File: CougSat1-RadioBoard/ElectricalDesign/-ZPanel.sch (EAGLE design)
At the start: 28 parts, among them J1 High Gain Antenna, J2 Deployables, J3 High Gain +, J4 ADCS, J5 Flap +X, J6 Flap -X, J7 Flap +Y, J8 Flap -Y, U1 LTC2499, U2 MCP1501-18

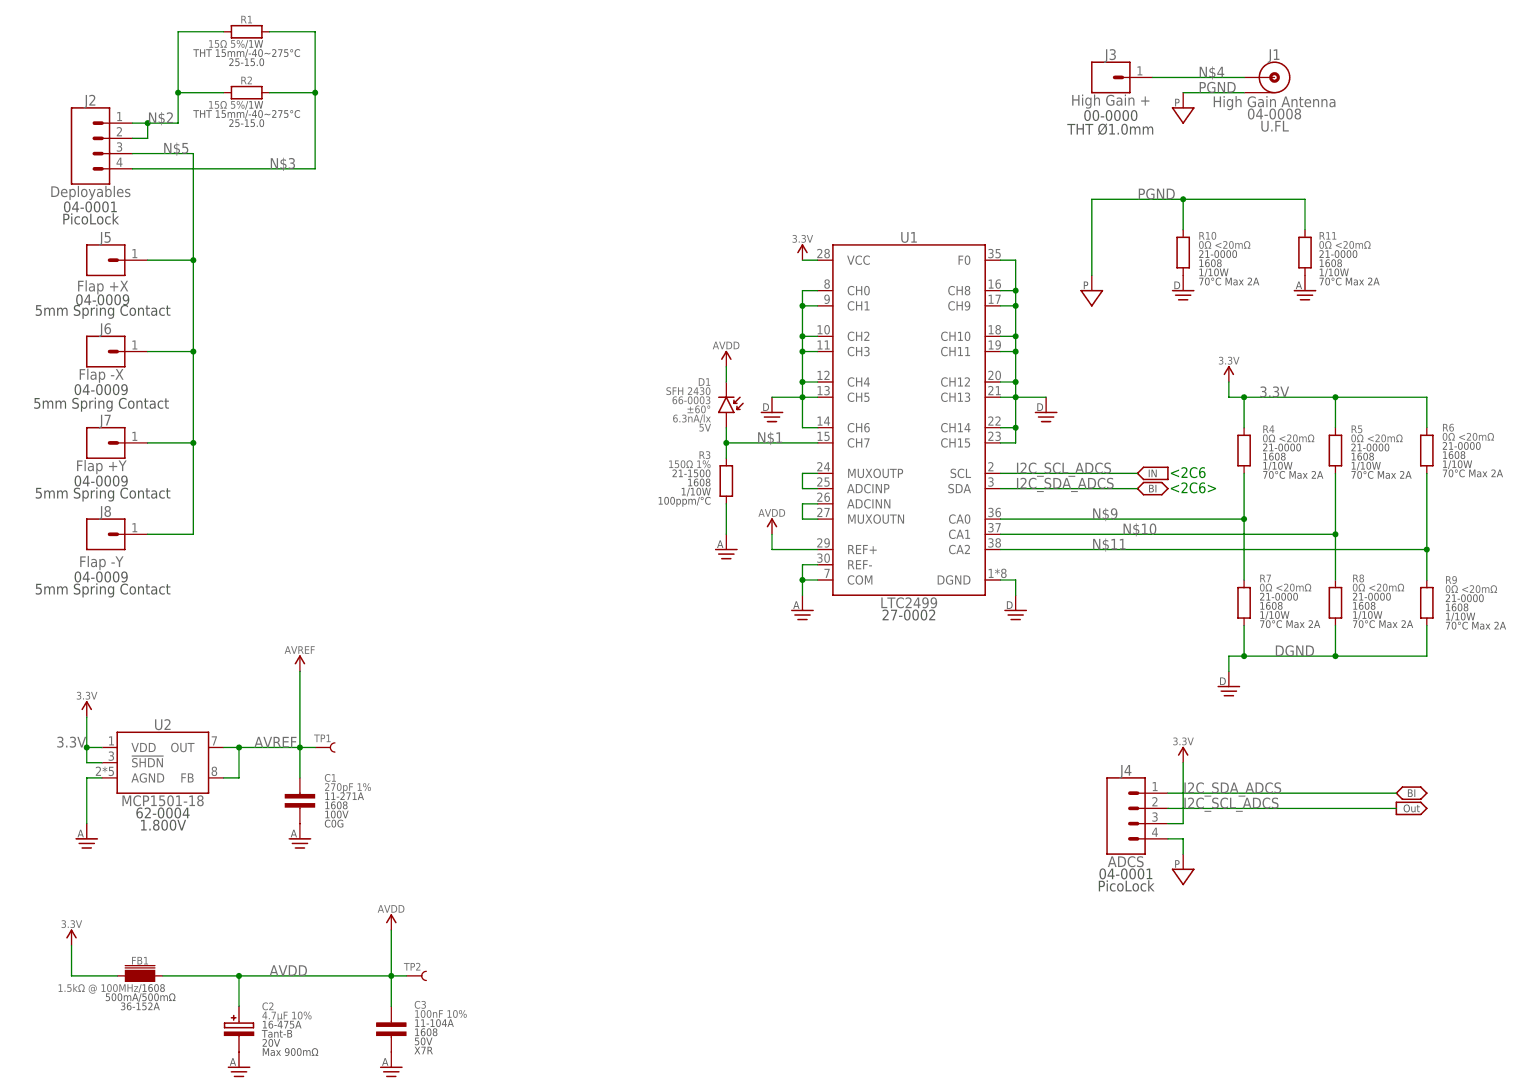
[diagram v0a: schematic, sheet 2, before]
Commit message: Update -ZPanel.sch
Ready for re-review
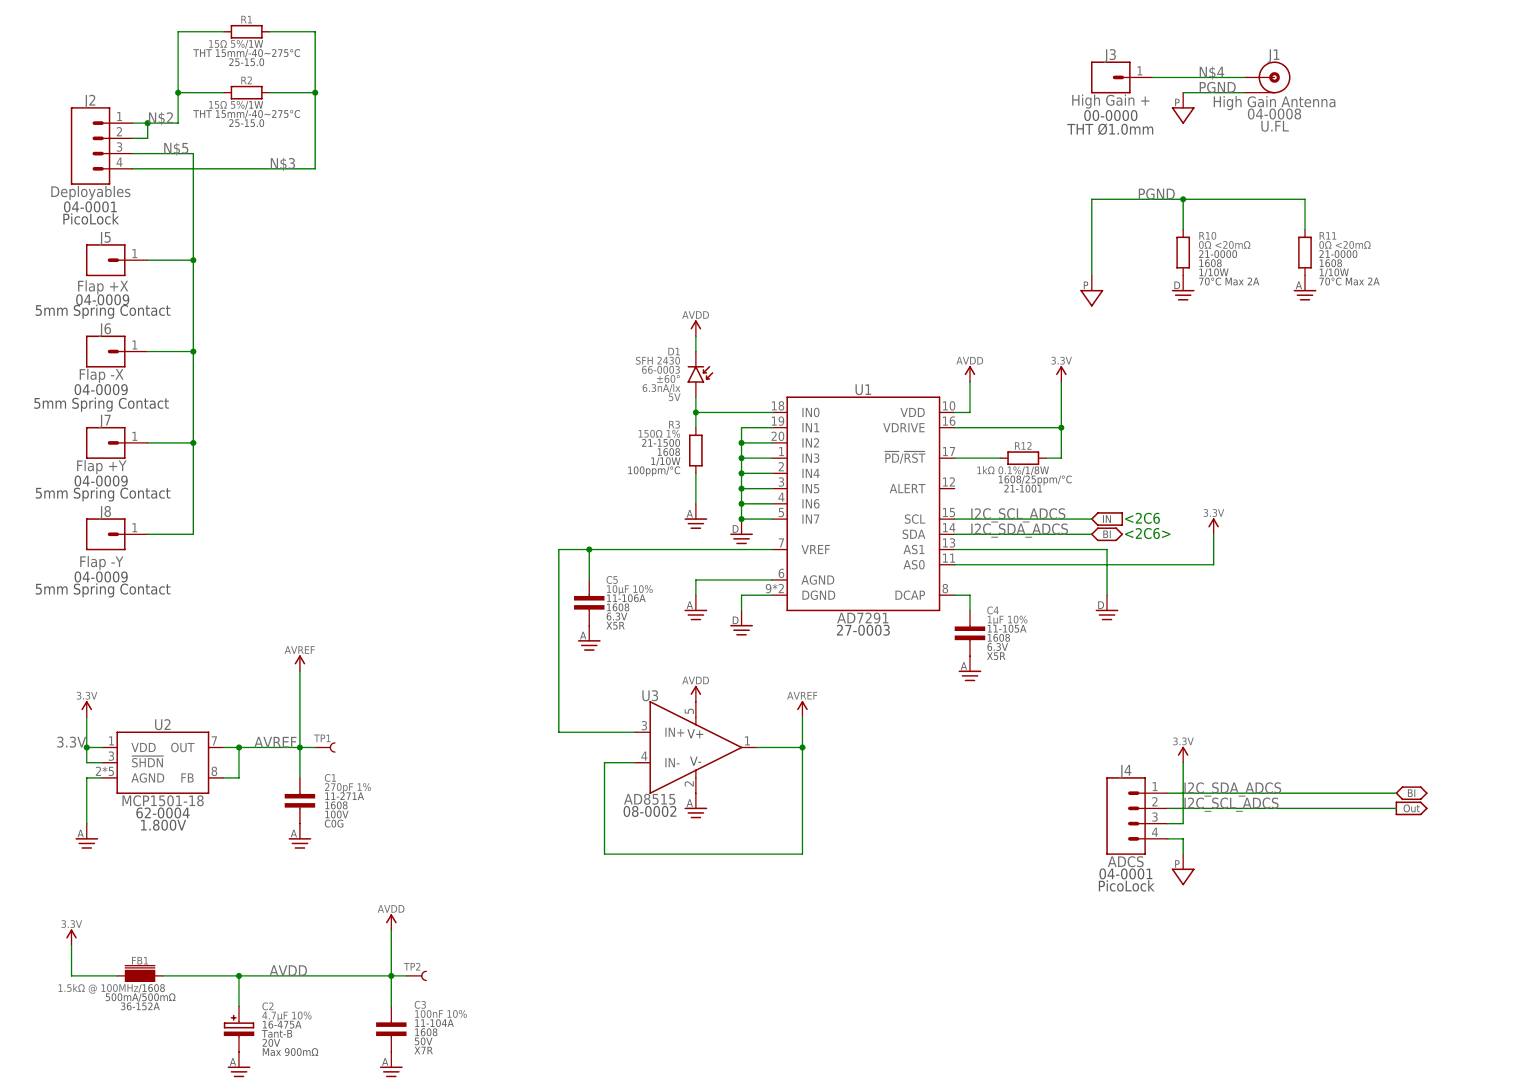
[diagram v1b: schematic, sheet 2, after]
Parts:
- removed R4, R5, R6, R7, R8, R9: 0Ω <20mΩ, CougsInSpace-Resistors:RES-V-0-1608
- added C4: 1µF 10%, CougsInSpace-Capacitors:CAP-V-1UF-1608
- added C5: 10µF 10%, CougsInSpace-Capacitors:CAP-V-10UF-1608
- added R12: 1kΩ 0.1%, CougsInSpace-Resistors:RES-H-1K-1608
- added U3: AD8515, CougsInSpace-IC-Amplifiers:OPAMP-1-AD8515
- U1: value LTC2499 -> AD7291; device CougsInSpace-IC-Conversion:LTC2499 -> CougsInSpace-IC-Conversion:AD7291
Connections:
- removed net N$10: R5.1, R8.2, U1.CA1
- removed net N$11: R6.1, R9.2, U1.CA2
- removed net N$7: U1.ADCINN, U1.MUXOUTN
- new net N$8: C4.1, U1.DCAP
- net 3.3V: now also R12.2, U1.AS0, U1.VDRIVE; no longer R4.2, R5.2, R6.2, U1.VCC
- net AGND: now also C4.2, C5.2, U1.AGND, U3.V-; no longer U1.COM, U1.REF-
- net AVDD: now also U1.VDD, U3.V+; no longer U1.REF+
- net AVREF: now also U3.IN-, U3.OUT
- net DGND: now also U1.AS1, U1.IN1, U1.IN2, U1.IN3, U1.IN4, U1.IN5, U1.IN6, U1.IN7; no longer R7.1, R8.1, R9.1, U1.CH0, U1.CH1, U1.CH10, U1.CH11, U1.CH12, U1.CH13, U1.CH14, U1.CH15, U1.CH2, U1.CH3, U1.CH4, U1.CH5, U1.CH6, U1.CH8, U1.CH9, U1.F0
- net N$1: now also U1.IN0; no longer U1.CH7
- net N$6: now also R12.1, U1.!PD!/!RST; no longer U1.ADCINP, U1.MUXOUTP
- net N$9: now also C5.1, U1.VREF, U3.IN+; no longer R4.1, R7.2, U1.CA0
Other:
- moved on the sheet: D1, R3
